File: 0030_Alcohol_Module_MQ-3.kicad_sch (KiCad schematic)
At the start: 11 parts, among them U1 MQ-3, U2 LM393D

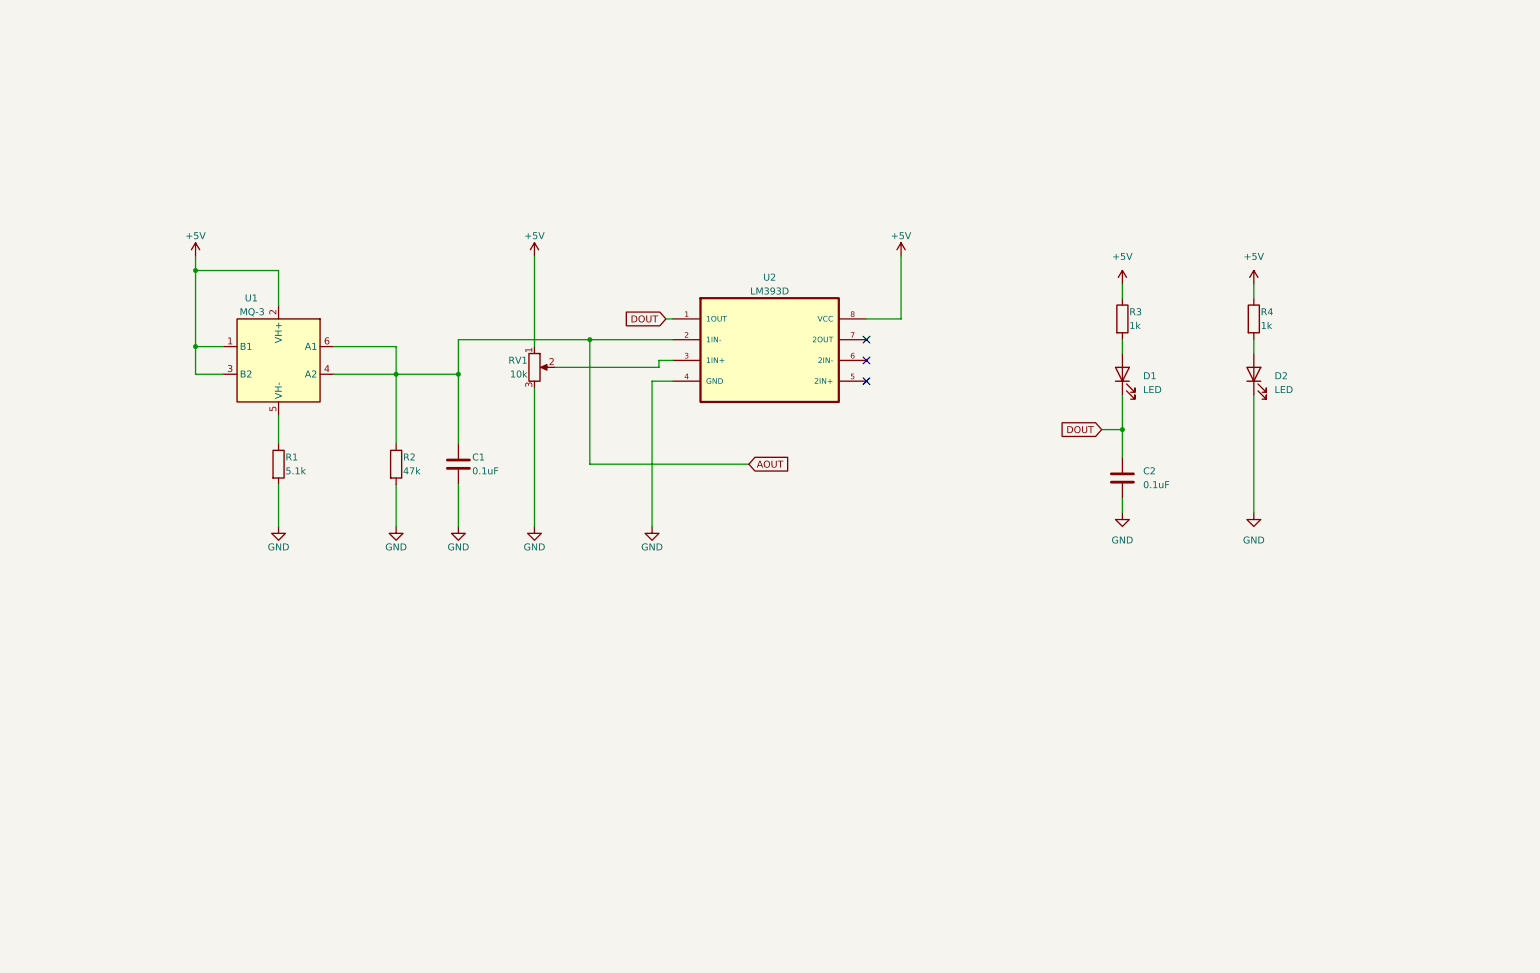
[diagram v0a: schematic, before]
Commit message: Add files via upload
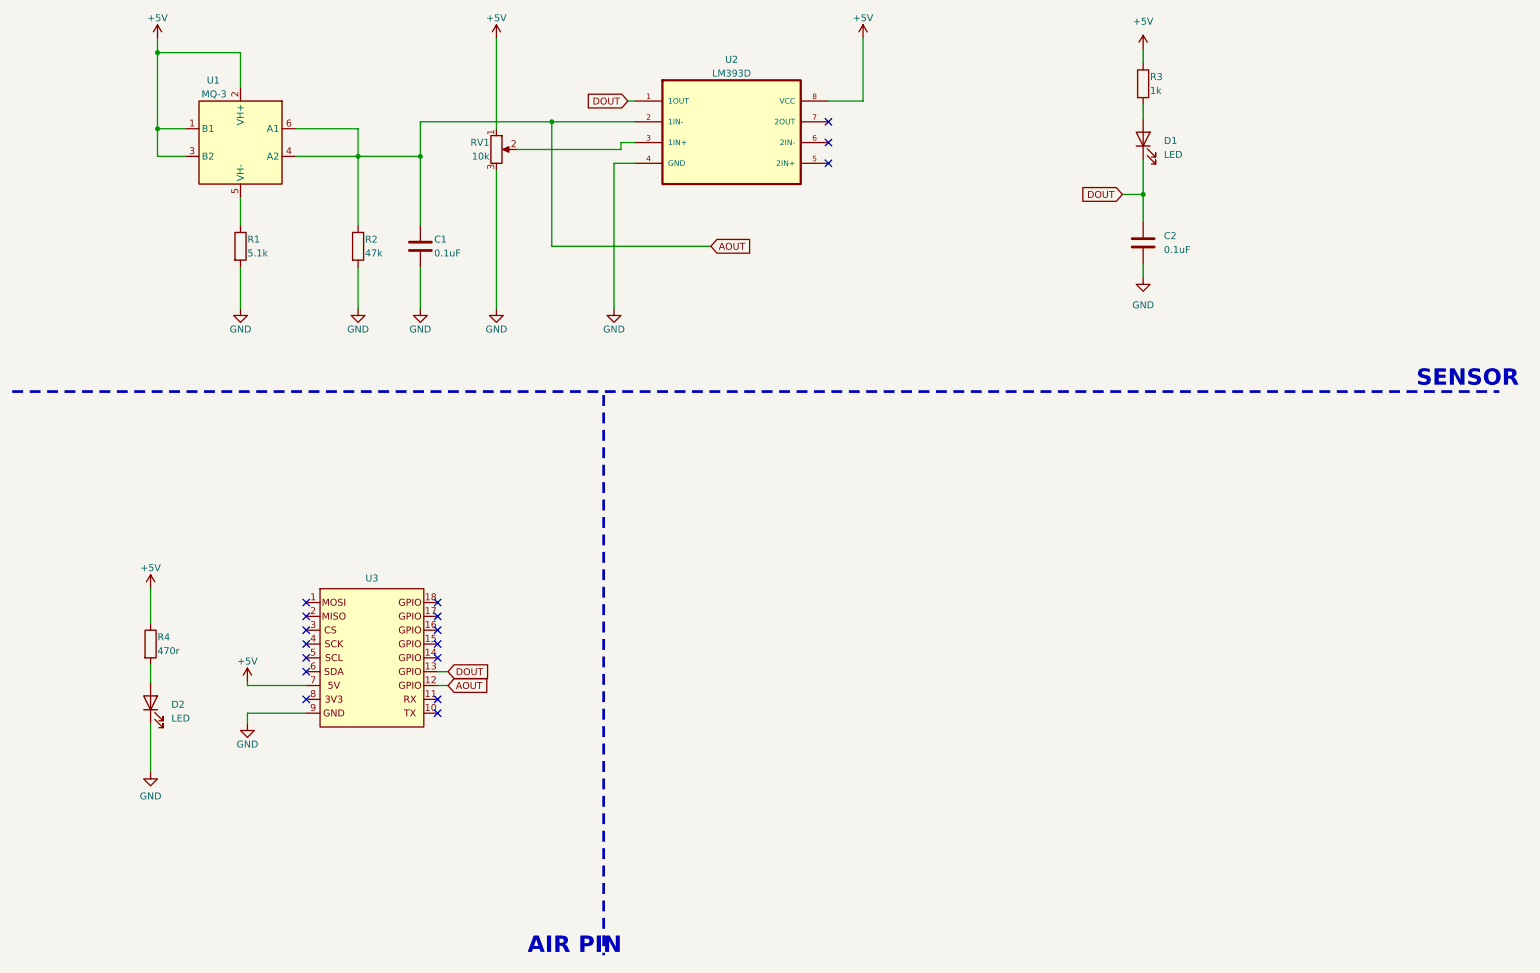
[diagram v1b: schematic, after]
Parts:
- added U3: ~, Moduler_:pin_header, symbol moduler_pin:air
- C1, C2: footprint (none) -> Capacitor_SMD:C_0805_2012Metric
- D1, D2: footprint (none) -> LED_SMD:LED_0805_2012Metric
- R1, R2, R3: footprint (none) -> Resistor_SMD:R_0805_2012Metric
- R4: value 1k -> 470r; footprint (none) -> Resistor_SMD:R_0805_2012Metric
- RV1: footprint (none) -> memin:3362P_1
- U2: footprint SOIC127P599X175-8N -> LM393:SOIC127P599X175-8N
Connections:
- net +5V: now also U3.7
- net AOUT: now also U3.12
- net DOUT: now also U3.13
- net GND: now also U3.9
- no-connect marks 3 -> 17
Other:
- note added: "AIR PIN"
- note added: "SENSOR"
- moved on the sheet: C1, C2, D1, D2, R1, R2, R3, R4, RV1, U1, U2
